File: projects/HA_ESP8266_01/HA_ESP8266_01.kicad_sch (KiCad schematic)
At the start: 17 parts, among them J1 IRQs, J2 DataPort A, J3 DataPort B, J4 PWR ext, J5 ~RESET, J6 I2C breakout, J7 D5-8 breakout, T1 HA-ESP8266-01, T2 (C)UweHerting, T3 https___github.com_uherting_M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, T4 v0.993, T5 JLCJLCJLCJLC, U1 NodeMCU V1, U2 I2C addr, U3 MCP23017M, U4 1WireBus, U5 1WireBus

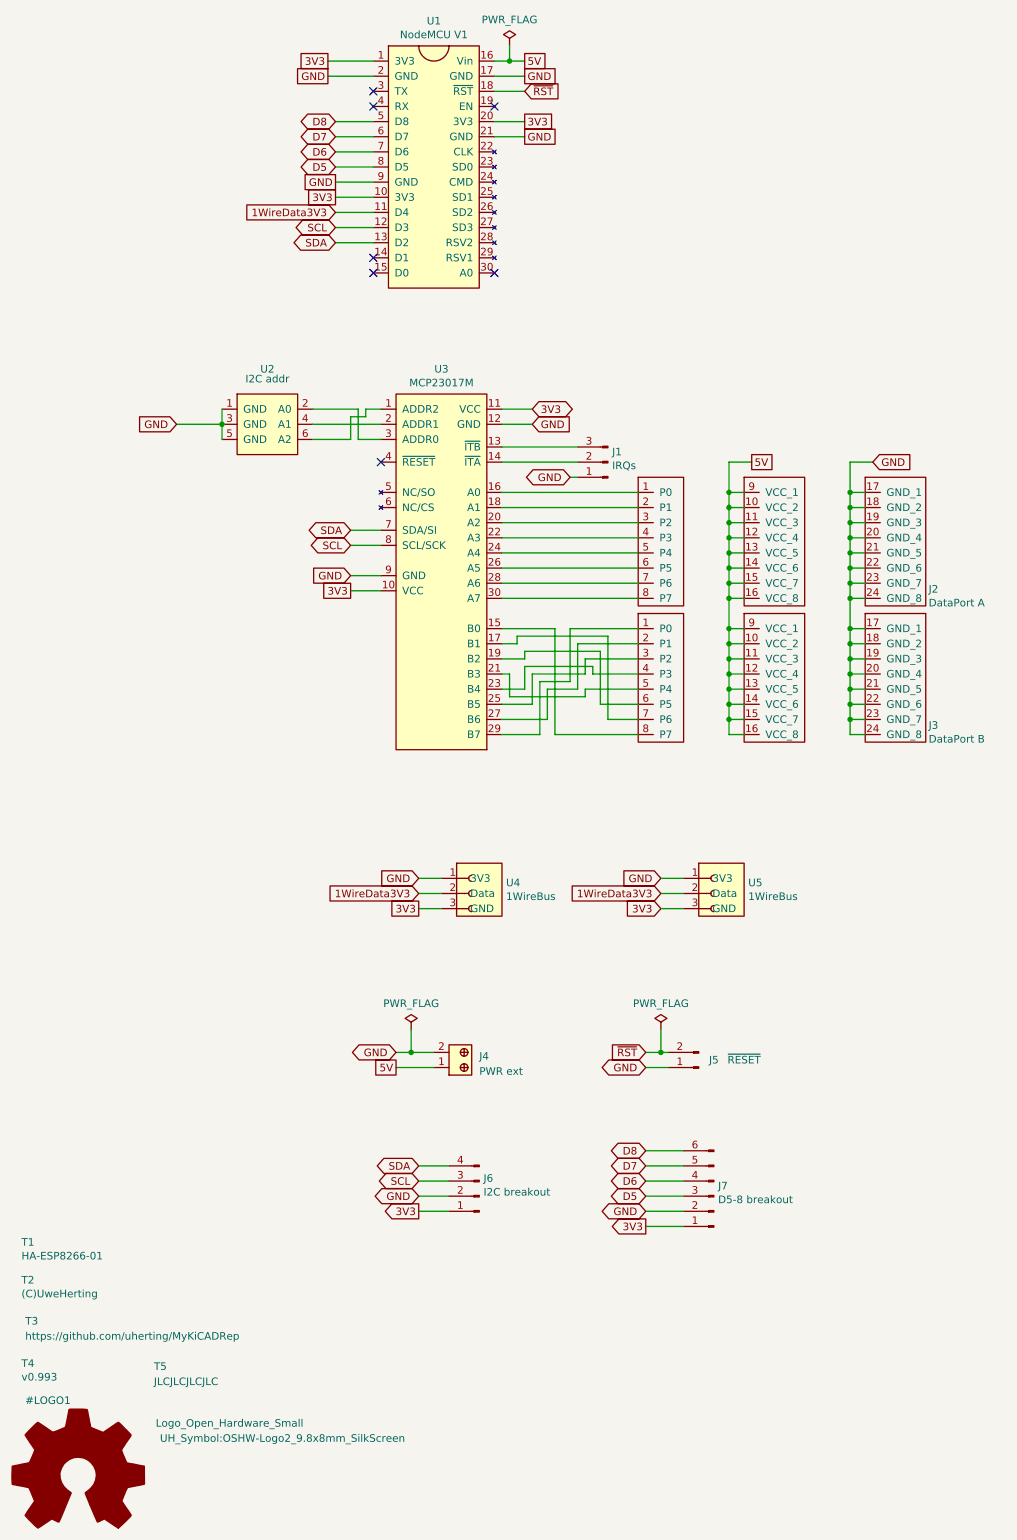
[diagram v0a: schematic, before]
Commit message: snapshot
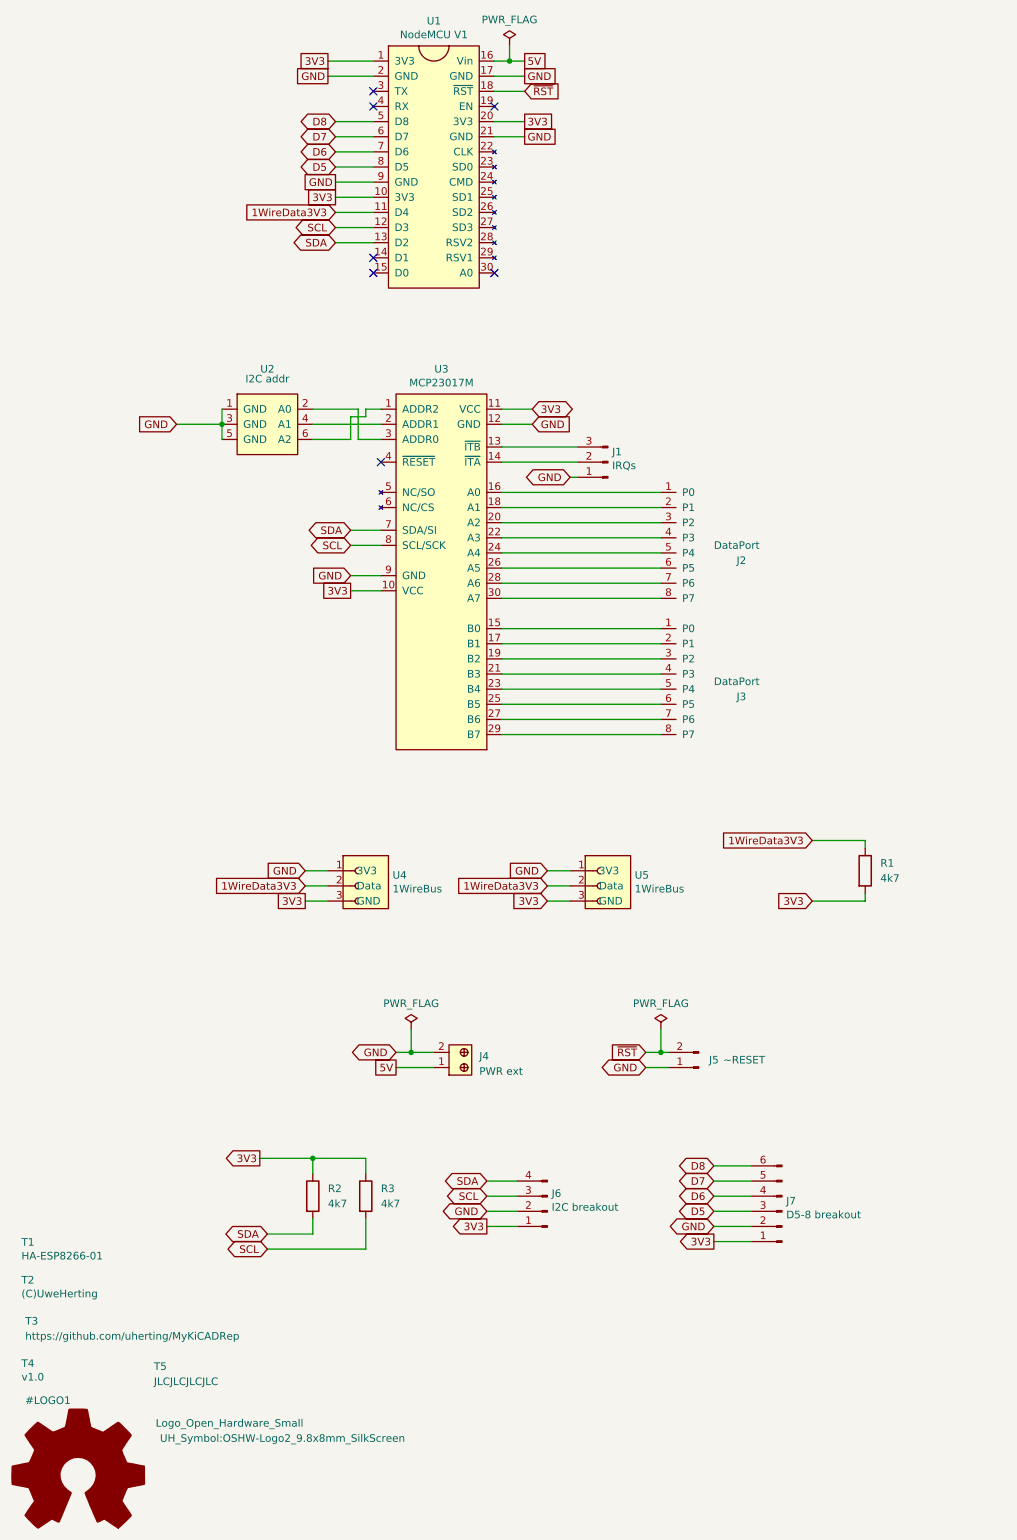
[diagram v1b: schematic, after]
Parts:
- removed J2: DataPort A, UH_HA:Dataport_WithPower, symbol UH_HA:DataPort_WithPower
- removed J3: DataPort B, UH_HA:Dataport_WithPower, symbol UH_HA:DataPort_WithPower
- added J2, J3: DataPort, UH_HA:PinHeader_1x08_P2.54mm_Vertical, symbol UH_HA:DataPort
- added R1, R2, R3: 4k7, UH_HA:R_0805_2012Metric_Pad1.20x1.40mm_HandSolder, symbol UH_HA:R
- T4: value v0.993 -> v1.0
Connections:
- net 1WireData3V3: now also R1.1
- net 3V3: now also R1.2, R2.1, R3.1
- net SCL: now also R3.2
- net SDA: now also R2.2
- net at U3.15 (B0): now also J3.1 (P0)
- net at U3.16 (A0): now also J2.1 (P0)
- net at U3.17 (B1): now also J3.2 (P1)
- net at U3.18 (A1): now also J2.2 (P1)
- net at U3.19 (B2): now also J3.3 (P2)
- net at U3.20 (A2): now also J2.3 (P2)
- net at U3.21 (B3): now also J3.4 (P3)
- net at U3.22 (A3): now also J2.4 (P3)
- net at U3.23 (B4): now also J3.5 (P4)
- net at U3.24 (A4): now also J2.5 (P4)
- net at U3.25 (B5): now also J3.6 (P5)
- net at U3.26 (A5): now also J2.6 (P5)
- net at U3.27 (B6): now also J3.7 (P6)
- net at U3.28 (A6): now also J2.7 (P6)
- net at U3.29 (B7): now also J3.8 (P7)
- net at U3.30 (A7): now also J2.8 (P7)
- net ~RST renamed ~{RST}
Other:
- moved on the sheet: J6, J7, U4, U5
